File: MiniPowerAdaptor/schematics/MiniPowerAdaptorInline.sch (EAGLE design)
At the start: 8 parts, among them IC1 LM317

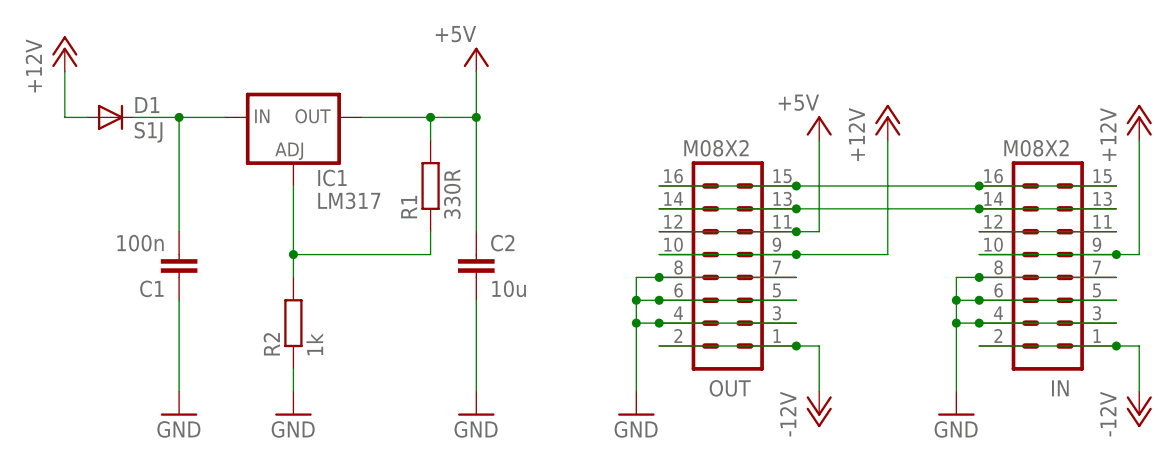
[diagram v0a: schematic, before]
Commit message: Rev03
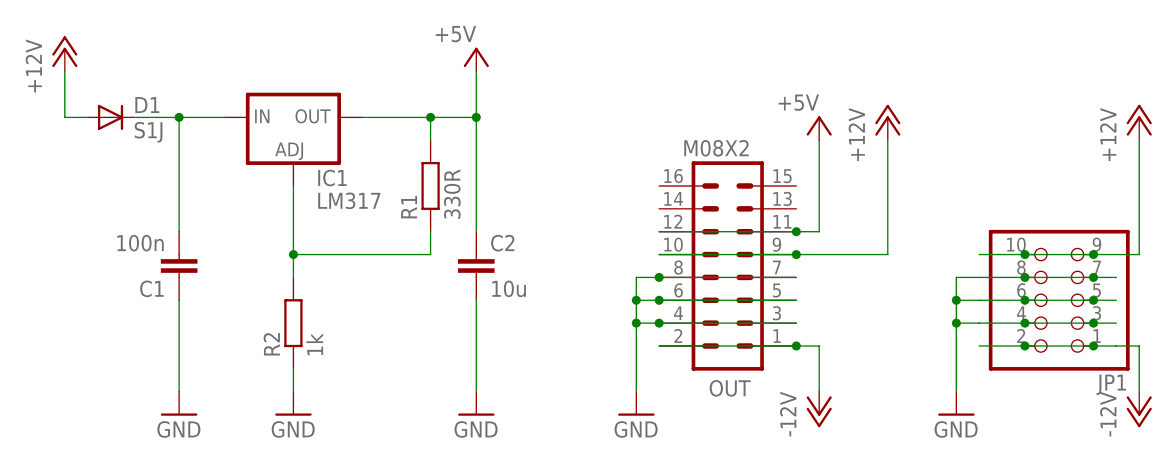
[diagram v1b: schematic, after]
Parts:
- removed IN: M08X2, SparkFun:M08X2
- added JP1: (no value), pinhead:PINHD-2X5
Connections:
- removed net N$2: IN.11, IN.12
- removed net N$4: IN.13, IN.14, OUT.13, OUT.14
- removed net N$5: IN.15, IN.16, OUT.15, OUT.16
- net +12V: now also JP1.10, JP1.9; no longer IN.10, IN.9
- net -12V: now also JP1.1, JP1.2; no longer IN.1, IN.2
- net GND: now also JP1.3, JP1.4, JP1.5, JP1.6, JP1.7, JP1.8; no longer IN.3, IN.4, IN.5, IN.6, IN.7, IN.8
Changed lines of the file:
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@@
 <?xml version="1.0" encoding="utf-8"?>
 <!DOCTYPE eagle SYSTEM "eagle.dtd">
-<eagle version="6.6.0">
+<eagle version="7.5.0">
 <drawing>
 <settings>
@@
 <part name="P+1" library="supply1" deviceset="+12V" device=""/>
 <part name="P+2" library="supply1" deviceset="+5V" device=""/>
-<part name="IN" library="SparkFun" deviceset="M08X2" device=""/>
 <part name="GND3" library="supply1" deviceset="GND" device=""/>
 <part name="P-1" library="supply1" deviceset="-12V" device=""/>
 <part name="P+3" library="supply1" deviceset="+12V" device=""/>
+<part name="JP1" library="pinhead" deviceset="PINHD-2X5" device=""/>
 </parts>
 <sheets>
@@
 <attribute name="VALUE" x="83.82" y="60.96" size="1.778" layer="96" rot="R180"/>
 </instance>
-<instance part="IN" gate="G$1" x="147.32" y="35.56" rot="R180"/>
 <instance part="GND3" gate="1" x="137.16" y="17.78"/>
 <instance part="P-1" gate="1" x="157.48" y="17.78"/>
 <instance part="P+3" gate="1" x="157.48" y="50.8"/>
+<instance part="JP1" gate="A" x="149.86" y="30.48" rot="R180"/>
 </instances>
 <busses>
@@
 </segment>
 <segment>
-<pinref part="IN" gate="G$1" pin="9"/>
 <pinref part="P+3" gate="1" pin="+12V"/>
 <wire x1="154.94" y1="35.56" x2="157.48" y2="35.56" width="0.1524" layer="91"/>
 <wire x1="157.48" y1="35.56" x2="157.48" y2="48.26" width="0.1524" layer="91"/>
-<pinref part="IN" gate="G$1" pin="10"/>
-<wire x1="139.7" y1="35.56" x2="154.94" y2="35.56" width="0.1524" layer="91"/>
-<junction x="154.94" y="35.56"/>
+<wire x1="139.7" y1="35.56" x2="144.78" y2="35.56" width="0.1524" layer="91"/>
+<pinref part="JP1" gate="A" pin="9"/>
+<wire x1="144.78" y1="35.56" x2="152.4" y2="35.56" width="0.1524" layer="91"/>
+<wire x1="152.4" y1="35.56" x2="154.94" y2="35.56" width="0.1524" layer="91"/>
+<junction x="152.4" y="35.56"/>
+<pinref part="JP1" gate="A" pin="10"/>
+<junction x="144.78" y="35.56"/>
 </segment>
 <segment>
@@
 </segment>
 <segment>
-<pinref part="IN" gate="G$1" pin="4"/>
 <pinref part="GND3" gate="1" pin="GND"/>
 <wire x1="139.7" y1="27.94" x2="137.16" y2="27.94" width="0.1524" layer="91"/>
 <wire x1="137.16" y1="27.94" x2="137.16" y2="20.32" width="0.1524" layer="91"/>
-<pinref part="IN" gate="G$1" pin="6"/>
 <wire x1="139.7" y1="30.48" x2="137.16" y2="30.48" width="0.1524" layer="91"/>
 <wire x1="137.16" y1="30.48" x2="137.16" y2="27.94" width="0.1524" layer="91"/>
 <junction x="137.16" y="27.94"/>
-<pinref part="IN" gate="G$1" pin="8"/>
 <wire x1="139.7" y1="33.02" x2="137.16" y2="33.02" width="0.1524" layer="91"/>
 <wire x1="137.16" y1="33.02" x2="137.16" y2="30.48" width="0.1524" layer="91"/>
 <junction x="137.16" y="30.48"/>
-<pinref part="IN" gate="G$1" pin="3"/>
-<wire x1="154.94" y1="27.94" x2="139.7" y2="27.94" width="0.1524" layer="91"/>
-<junction x="139.7" y="27.94"/>
-<pinref part="IN" gate="G$1" pin="5"/>
-<wire x1="139.7" y1="30.48" x2="154.94" y2="30.48" width="0.1524" layer="91"/>
-<junction x="139.7" y="30.48"/>
-<pinref part="IN" gate="G$1" pin="7"/>
-<wire x1="139.7" y1="33.02" x2="154.94" y2="33.02" width="0.1524" layer="91"/>
-<junction x="139.7" y="33.02"/>
+<wire x1="154.94" y1="27.94" x2="152.4" y2="27.94" width="0.1524" layer="91"/>
+<wire x1="152.4" y1="27.94" x2="144.78" y2="27.94" width="0.1524" layer="91"/>
+<wire x1="144.78" y1="27.94" x2="139.7" y2="27.94" width="0.1524" layer="91"/>
+<wire x1="139.7" y1="30.48" x2="144.78" y2="30.48" width="0.1524" layer="91"/>
+<wire x1="144.78" y1="30.48" x2="152.4" y2="30.48" width="0.1524" layer="91"/>
+<wire x1="152.4" y1="30.48" x2="154.94" y2="30.48" width="0.1524" layer="91"/>
+<wire x1="139.7" y1="33.02" x2="144.78" y2="33.02" width="0.1524" layer="91"/>
+<pinref part="JP1" gate="A" pin="3"/>
+<junction x="152.4" y="27.94"/>
+<pinref part="JP1" gate="A" pin="4"/>
+<junction x="144.78" y="27.94"/>
+<pinref part="JP1" gate="A" pin="5"/>
+<junction x="152.4" y="30.48"/>
+<pinref part="JP1" gate="A" pin="6"/>
+<junction x="144.78" y="30.48"/>
+<pinref part="JP1" gate="A" pin="7"/>
+<wire x1="144.78" y1="33.02" x2="152.4" y2="33.02" width="0.1524" layer="91"/>
+<wire x1="152.4" y1="33.02" x2="154.94" y2="33.02" width="0.1524" layer="91"/>
+<junction x="152.4" y="33.02"/>
+<pinref part="JP1" gate="A" pin="8"/>
+<junction x="144.78" y="33.02"/>
 </segment>
 </net>
 <net name="-12V" class="0">
 <segment>
-<pinref part="IN" gate="G$1" pin="1"/>
 <pinref part="P-1" gate="1" pin="-12V"/>
 <wire x1="154.94" y1="25.4" x2="157.48" y2="25.4" width="0.1524" layer="91"/>
 <wire x1="157.48" y1="25.4" x2="157.48" y2="20.32" width="0.1524" layer="91"/>
-<pinref part="IN" gate="G$1" pin="2"/>
-<wire x1="139.7" y1="25.4" x2="154.94" y2="25.4" width="0.1524" layer="91"/>
-<junction x="154.94" y="25.4"/>
+<wire x1="139.7" y1="25.4" x2="144.78" y2="25.4" width="0.1524" layer="91"/>
+<pinref part="JP1" gate="A" pin="1"/>
+<wire x1="144.78" y1="25.4" x2="152.4" y2="25.4" width="0.1524" layer="91"/>
+<wire x1="152.4" y1="25.4" x2="154.94" y2="25.4" width="0.1524" layer="91"/>
+<junction x="152.4" y="25.4"/>
+<pinref part="JP1" gate="A" pin="2"/>
+<junction x="144.78" y="25.4"/>
 </segment>
 <segment>
@@
 </segment>
 </net>
-<net name="N$2" class="0">
-<segment>
-<pinref part="IN" gate="G$1" pin="12"/>
-<pinref part="IN" gate="G$1" pin="11"/>
-<wire x1="139.7" y1="38.1" x2="154.94" y2="38.1" width="0.1524" layer="91"/>
-</segment>
-</net>
-<net name="N$4" class="0">
-<segment>
-<pinref part="OUT" gate="G$1" pin="14"/>
-<pinref part="OUT" gate="G$1" pin="13"/>
-<wire x1="104.14" y1="40.64" x2="119.38" y2="40.64" width="0.1524" layer="91"/>
-<pinref part="IN" gate="G$1" pin="14"/>
-<wire x1="119.38" y1="40.64" x2="139.7" y2="40.64" width="0.1524" layer="91"/>
-<junction x="119.38" y="40.64"/>
-<pinref part="IN" gate="G$1" pin="13"/>
-<wire x1="154.94" y1="40.64" x2="139.7" y2="40.64" width="0.1524" layer="91"/>
-<junction x="139.7" y="40.64"/>
-</segment>
-</net>
-<net name="N$5" class="0">
-<segment>
-<pinref part="IN" gate="G$1" pin="15"/>
-<pinref part="IN" gate="G$1" pin="16"/>
-<wire x1="154.94" y1="43.18" x2="139.7" y2="43.18" width="0.1524" layer="91"/>
-<pinref part="OUT" gate="G$1" pin="15"/>
-<wire x1="139.7" y1="43.18" x2="119.38" y2="43.18" width="0.1524" layer="91"/>
-<junction x="139.7" y="43.18"/>
-<pinref part="OUT" gate="G$1" pin="16"/>
-<wire x1="119.38" y1="43.18" x2="104.14" y2="43.18" width="0.1524" layer="91"/>
-<junction x="119.38" y="43.18"/>
-</segment>
-</net>
